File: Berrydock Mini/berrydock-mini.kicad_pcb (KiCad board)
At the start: 2 copper layers, 50 x 50 mm, 88 parts, among them J1 RJ45, P1 CONN_01X16, P2 CONN_01X07, P3 CONN_01X04, P4 CONN_01X03, P5 USB_OTG, P6 USB_A, SW1 SWITCH_INV, SW2 BUTTON, U1 CP2102, U10 L6920DC, U11 FS8205A, U12 DW01-P, U13 USBLC6-2, U14 USBLC6-2, U3 TD6811, U4 H1260NL, U5 Omega2, U8 ACT4088, U9 MCP73831

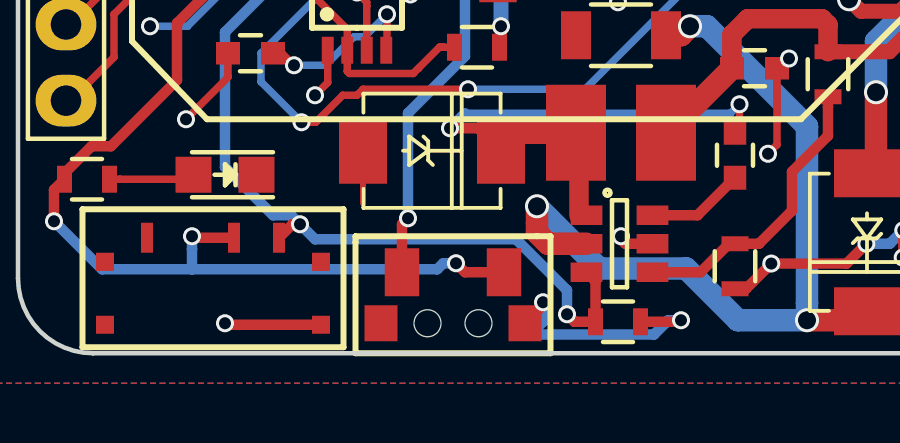
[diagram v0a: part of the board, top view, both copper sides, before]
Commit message: updates in pcb
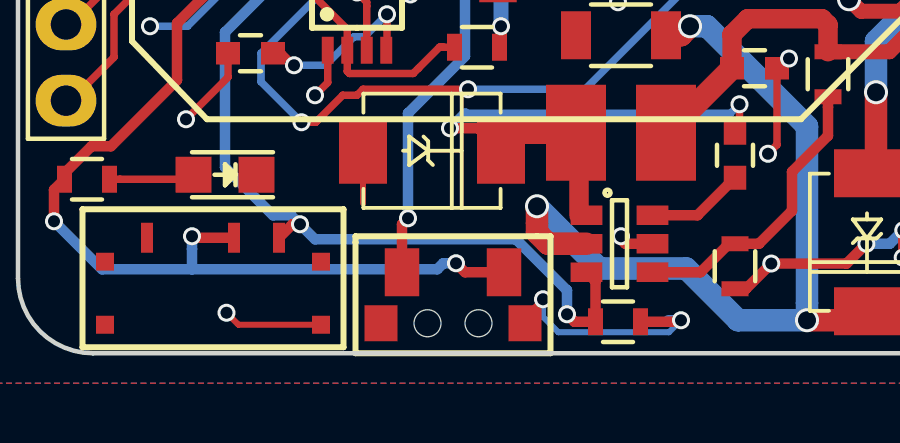
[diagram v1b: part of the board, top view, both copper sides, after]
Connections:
- SW1 pad 4: (no net) -> GND
- SW2 pad 3: (no net) -> GND
- SW2 pad 4: (no net) -> GND
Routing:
- net (no net): track 3.22 -> 0.00 mm, vias 1 -> 0
- net GND: track 225.2 -> 228.1 mm, vias 64 -> 65
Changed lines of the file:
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@@
 (kicad_pcb (version 4) (host pcbnew 4.0.3-stable)
   (general
-    (links 208)
+    (links 214)
     (no_connects 0)
-    (area 19.924999 19.924999 70.075001 70.075001)
+    (area 16.566667 17.16246 71.975 74.875)
     (thickness 1.6)
     (drawings 14)
-    (tracks 1670)
+    (tracks 1669)
     (zones 0)
     (modules 88)
@@
   (page A4)
   (layers
-    (0 F.Cu signal hide)
-    (31 B.Cu signal hide)
+    (0 F.Cu signal)
+    (31 B.Cu signal)
     (32 B.Adhes user)
     (33 F.Adhes user)
@@
     (pad_to_mask_clearance 0.2)
     (aux_axis_origin 0 0)
-    (visible_elements 7FFFF97F)
+    (grid_origin 20 20)
+    (visible_elements 7FFFFF7F)
     (pcbplotparams
       (layerselection 0x010f0_80000001)
@@
       (psnegative false)
       (psa4output false)
-      (plotreference true)
+      (plotreference false)
       (plotvalue false)
       (plotinvisibletext false)
@@
     (pad 3 smd rect (at 2.2 1.85 180) (size 0.4 1) (layers F.Cu F.Paste F.Mask)
       (net 77 "Net-(SW1-Pad3)"))
-    (pad 4 smd rect (at 3.6 1.05 180) (size 0.6 0.6) (layers F.Cu F.Paste F.Mask))
-    (pad 4 smd rect (at 3.6 -1.05 180) (size 0.6 0.6) (layers F.Cu F.Paste F.Mask))
-    (pad 4 smd rect (at -3.6 -1.05 180) (size 0.6 0.6) (layers F.Cu F.Paste F.Mask))
-    (pad 4 smd rect (at -3.6 1.05 180) (size 0.6 0.6) (layers F.Cu F.Paste F.Mask))
+    (pad 4 smd rect (at 3.6 1.05 180) (size 0.6 0.6) (layers F.Cu F.Paste F.Mask)
+      (net 2 GND))
+    (pad 4 smd rect (at 3.6 -1.05 180) (size 0.6 0.6) (layers F.Cu F.Paste F.Mask)
+      (net 2 GND))
+    (pad 4 smd rect (at -3.6 -1.05 180) (size 0.6 0.6) (layers F.Cu F.Paste F.Mask)
+      (net 2 GND))
+    (pad 4 smd rect (at -3.6 1.05 180) (size 0.6 0.6) (layers F.Cu F.Paste F.Mask)
+      (net 2 GND))
   )
   (module Omega2-Berrydock:SMD-BUTTON-2x4x3,5 (layer F.Cu)
@@
     (pad 2 smd rect (at 1.7 1.7 180) (size 1.15 1.6) (layers F.Cu F.Paste F.Mask)
       (net 67 "Net-(R27-Pad2)"))
-    (pad 3 smd rect (at 2.4 0 180) (size 1.1 1.2) (layers F.Cu F.Paste F.Mask))
-    (pad 4 smd rect (at -2.4 0 180) (size 1.1 1.2) (layers F.Cu F.Paste F.Mask))
+    (pad 3 smd rect (at 2.4 0 180) (size 1.1 1.2) (layers F.Cu F.Paste F.Mask)
+      (net 2 GND))
+    (pad 4 smd rect (at -2.4 0 180) (size 1.1 1.2) (layers F.Cu F.Paste F.Mask)
+      (net 2 GND))
     (pad "" np_thru_hole circle (at -0.85 0 180) (size 0.9 0.9) (drill 0.9) (layers *.Cu *.Mask))
     (pad "" np_thru_hole circle (at 0.85 0 180) (size 0.9 0.9) (drill 0.9) (layers *.Cu *.Mask))
@@
   (gr_line (start 20 67.5) (end 20 22.5) (angle 90) (layer Edge.Cuts) (width 0.15))
   (gr_line (start 67.5 70) (end 22.5 70) (angle 90) (layer Edge.Cuts) (width 0.15))
-  (segment (start 30.1 69.05) (end 26.95 69.05) (width 0.35) (layer F.Cu) (net 0))
-  (segment (start 26.95 69.05) (end 26.9 69) (width 0.35) (layer F.Cu) (net 0))
-  (via (at 26.9 69) (size 0.6) (drill 0.4) (layers F.Cu B.Cu) (net 0))
   (segment (start 35.5 36.2) (end 35.5 37.55219) (width 0.35) (layer F.Cu) (net 1))
   (segment (start 35.5 37.55219) (end 35.258698 37.793492) (width 0.35) (layer F.Cu) (net 1))
@@
   (segment (start 37.996198 39.255992) (end 37.996198 38.980992) (width 0.25) (layer F.Cu) (net 1))
   (segment (start 37.996198 38.980992) (end 37.2 38.184794) (width 0.25) (layer F.Cu) (net 1))
+  (segment (start 37.5 68.2) (end 37.5 68.788002) (width 0.2) (layer B.Cu) (net 2))
+  (segment (start 37.5 68.788002) (end 38.011999 69.300001) (width 0.2) (layer B.Cu) (net 2))
+  (segment (start 38.011999 69.300001) (end 41.699999 69.300001) (width 0.2) (layer B.Cu) (net 2))
+  (via (at 42.1 68.9) (size 0.6) (drill 0.4) (layers F.Cu B.Cu) (net 2))
+  (segment (start 41.699999 69.300001) (end 42.1 68.9) (width 0.2) (layer B.Cu) (net 2))
+  (segment (start 36.9 69) (end 36.9 68.8) (width 0.2) (layer F.Cu) (net 2))
+  (segment (start 36.9 68.8) (end 37.5 68.2) (width 0.2) (layer F.Cu) (net 2))
+  (via (at 37.5 68.2) (size 0.6) (drill 0.4) (layers F.Cu B.Cu) (net 2))
+  (segment (start 30.1 69.05) (end 27.35 69.05) (width 0.2) (layer F.Cu) (net 2))
+  (segment (start 27.35 69.05) (end 26.95 68.65) (width 0.2) (layer F.Cu) (net 2))
+  (via (at 26.95 68.65) (size 0.6) (drill 0.4) (layers F.Cu B.Cu) (net 2))
   (segment (start 40.1 66.1) (end 40.1 66.2) (width 0.35) (layer F.Cu) (net 2))
   (segment (start 40.1 66.2) (end 40.25 66.35) (width 0.35) (layer F.Cu) (net 2))
-  (segment (start 37.5 68.3) (end 37.5 68.4) (width 0.35) (layer F.Cu) (net 2))
-  (segment (start 37.5 68.4) (end 36.9 69) (width 0.35) (layer F.Cu) (net 2))
-  (segment (start 37.075001 69.375001) (end 37.5 68.950002) (width 0.35) (layer B.Cu) (net 2))
-  (segment (start 37.5 68.950002) (end 37.5 68.3) (width 0.35) (layer B.Cu) (net 2))
-  (via (at 37.5 68.3) (size 0.6) (drill 0.4) (layers F.Cu B.Cu) (net 2))
-  (segment (start 41.575736 69) (end 41.200735 69.375001) (width 0.35) (layer B.Cu) (net 2))
-  (segment (start 41.200735 69.375001) (end 37.075001 69.375001) (width 0.35) (layer B.Cu) (net 2))
   (segment (start 42.1 68.9) (end 41.675736 68.9) (width 0.35) (layer B.Cu) (net 2))
-  (segment (start 41.675736 68.9) (end 41.575736 69) (width 0.35) (layer B.Cu) (net 2))
   (segment (start 40.75 68.95) (end 42.05 68.95) (width 0.35) (layer F.Cu) (net 2))
   (segment (start 42.05 68.95) (end 42.1 68.9) (width 0.35) (layer F.Cu) (net 2))
-  (via (at 42.1 68.9) (size 0.6) (drill 0.4) (layers F.Cu B.Cu) (net 2))
   (segment (start 65.45 34.85) (end 65.5 34.85) (width 0.2) (layer B.Cu) (net 2))
   (segment (start 65.5 34.85) (end 66.65 33.7) (width 0.2) (layer B.Cu) (net 2))
